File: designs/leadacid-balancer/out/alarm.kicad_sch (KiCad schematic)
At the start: 1 part, among them J2 1757242

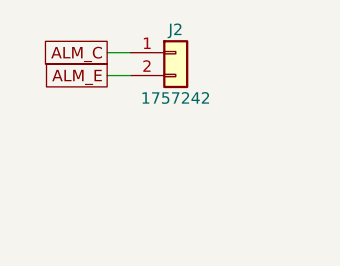
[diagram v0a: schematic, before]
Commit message: designs: work-in-progress (review fixes under way)
Co-Authored-By: Claude Opus 5.5 <noreply@anthropic.com>
Claude-Session: https://claude.ai/code/session_01VFJn9VbX8h27kf4LpLwEtn
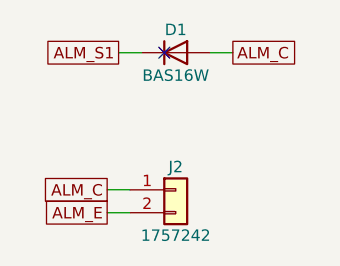
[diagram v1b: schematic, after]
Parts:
- added D1: BAS16W, Package_TO_SOT_SMD:SOT-323_SC-70, symbol Diode:BAS16W
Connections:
- net ALM_C: now also D1.1 (A)
- new net ALM_S1: D1.3 (K)
- no-connect marks 0 -> 1
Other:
- moved on the sheet: J2
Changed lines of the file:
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@@
 		(rev "A")
 		(company "kaesynth")
-		(comment 1 "J2 = MSTBA 2-pos: 1 ALM_C, 2 ALM_E; U110/U210/U310 collectors in parallel")
+		(comment 1 "J2 = MSTBA 2-pos: 1 ALM_C, 2 ALM_E; D1 blocks a reversed loop (review MINOR-9); U110, U210, U310 outputs in series: closed = healthy (fail-safe)")
 		(comment 2 "Lead-acid string balancer, 2:1 switched capacitor, 2-4 x 12 V — generated by kaesynth from design.py; do not edit by hand")
 	)
 	(symbol
 		(lib_id "Connector_Generic:Conn_01x02")
+		(at 43.18 45.72 0)
+		(unit 1)
+		(exclude_from_sim no)
+		(in_bom yes)
+		(on_board yes)
+		(dnp no)
+		(property "Reference" "J2"
+			(at 43.18 43.18 0)
+			(effects
+				(font (size 1.27 1.27))
+			)
+		)
+		(property "Value" "1757242"
+			(at 43.18 50.8 0)
+			(effects
+				(font (size 1.27 1.27))
+			)
+		)
+		(property "Footprint" "Connector_Phoenix_MSTB:PhoenixContact_MSTBA_2,5_2-G-5,08_1x02_P5.08mm_Horizontal"
+			(at 43.18 45.72 0)
+			(hide yes)
+			(effects
+				(font (size 1.27 1.27))
+			)
+		)
+		(property "Datasheet" "https://www.phoenixcontact.com/en-us/products/pcb-header-mstba-25-2-g-508-1757242"
+			(at 43.18 45.72 0)
+			(hide yes)
+			(effects
+				(font (size 1.27 1.27))
+			)
+		)
+		(property "Description" "PCB header MSTBA 2,5/2-G-5,08, 2 pos (isolated alarm contact)"
+			(at 43.18 45.72 0)
+			(hide yes)
+			(effects
+				(font (size 1.27 1.27))
+			)
+		)
+		(property "MPN" "1757242"
+			(at 43.18 45.72 0)
+			(hide yes)
+			(effects
+				(font (size 1.27 1.27))
+			)
+		)
+		(property "Manufacturer" "Phoenix Contact"
+			(at 43.18 45.72 0)
+			(hide yes)
+			(effects
+				(font (size 1.27 1.27))
+			)
+		)
+		(property "Block" "alarm"
+			(at 43.18 45.72 0)
+			(hide yes)
+			(effects
+				(font (size 1.27 1.27))
+			)
+		)
+		(property "Component Class" "alarm"
+			(at 43.18 45.72 0)
+			(hide yes)
+			(effects
+				(font (size 1.27 1.27))
+			)
+		)
+		(pin "1"
+		)
+		(pin "2"
+		)
+		(instances
+			(project "leadacid-balancer"
+				(path "/19cb7a1a-0065-5673-9954-2860fa0f563d/cf1d326d-1904-5168-b9da-d8ce55ede38b"
+					(reference "J2")
+					(unit 1)
+				)
+			)
+		)
+	)
+	(wire
+		(pts (xy 38.1 45.72) (xy 35.56 45.72))
+		(stroke
+			(width 0)
+			(type default)
+		)
+	)
+	(global_label "ALM_C"
+		(shape passive)
+		(at 35.56 45.72 180)
+		(fields_autoplaced yes)
+		(effects
+			(font (size 1.27 1.27))
+			(justify right)
+		)
+		(property "Intersheetrefs" "${INTERSHEET_REFS}"
+			(at 35.56 45.72 0)
+			(hide yes)
+			(effects
+				(font (size 1.27 1.27))
+			)
+		)
+	)
+	(wire
+		(pts (xy 38.1 48.26) (xy 35.56 48.26))
+		(stroke
+			(width 0)
+			(type default)
+		)
+	)
+	(global_label "ALM_E"
+		(shape passive)
+		(at 35.56 48.26 180)
+		(fields_autoplaced yes)
+		(effects
+			(font (size 1.27 1.27))
+			(justify right)
+		)
+		(property "Intersheetrefs" "${INTERSHEET_REFS}"
+			(at 35.56 48.26 0)
+			(hide yes)
+			(effects
+				(font (size 1.27 1.27))
+			)
+		)
+	)
+	(symbol
+		(lib_id "Diode:BAS16W")
 		(at 43.18 30.48 0)
 		(unit 1)
@@
 		(on_board yes)
 		(dnp no)
-		(property "Reference" "J2"
+		(property "Reference" "D1"
 			(at 43.18 27.94 0)
 			(effects
@@
 			)
 		)
-		(property "Value" "1757242"
-			(at 43.18 35.56 0)
-			(effects
-				(font (size 1.27 1.27))
-			)
-		)
-		(property "Footprint" "Connector_Phoenix_MSTB:PhoenixContact_MSTBA_2,5_2-G-5,08_1x02_P5.08mm_Horizontal"
-			(at 43.18 30.48 0)
-			(hide yes)
-			(effects
-				(font (size 1.27 1.27))
-			)
-		)
-		(property "Datasheet" "https://www.phoenixcontact.com/en-us/products/pcb-header-mstba-25-2-g-508-1757242"
-			(at 43.18 30.48 0)
-			(hide yes)
-			(effects
-				(font (size 1.27 1.27))
-			)
-		)
-		(property "Description" "PCB header MSTBA 2,5/2-G-5,08, 2 pos (isolated alarm contact)"
-			(at 43.18 30.48 0)
-			(hide yes)
-			(effects
-				(font (size 1.27 1.27))
-			)
-		)
-		(property "MPN" "1757242"
-			(at 43.18 30.48 0)
-			(hide yes)
-			(effects
-				(font (size 1.27 1.27))
-			)
-		)
-		(property "Manufacturer" "Phoenix Contact"
+		(property "Value" "BAS16W"
+			(at 43.18 33.02 0)
+			(effects
+				(font (size 1.27 1.27))
+			)
+		)
+		(property "Footprint" "Package_TO_SOT_SMD:SOT-323_SC-70"
+			(at 43.18 30.48 0)
+			(hide yes)
+			(effects
+				(font (size 1.27 1.27))
+			)
+		)
+		(property "Datasheet" "https://www.diodes.com/assets/Datasheets/ds30117.pdf"
+			(at 43.18 30.48 0)
+			(hide yes)
+			(effects
+				(font (size 1.27 1.27))
+			)
+		)
+		(property "Description" "Switching diode 75 V 150 mA SOT-323 (bootstrap)"
+			(at 43.18 30.48 0)
+			(hide yes)
+			(effects
+				(font (size 1.27 1.27))
+			)
+		)
+		(property "MPN" "BAS16W-7-F"
+			(at 43.18 30.48 0)
+			(hide yes)
+			(effects
+				(font (size 1.27 1.27))
+			)
+		)
+		(property "Manufacturer" "Diodes Incorporated"
 			(at 43.18 30.48 0)
 			(hide yes)
@@
 		)
 		(pin "2"
+		)
+		(pin "3"
 		)
 		(instances
 			(project "leadacid-balancer"
 				(path "/19cb7a1a-0065-5673-9954-2860fa0f563d/cf1d326d-1904-5168-b9da-d8ce55ede38b"
-					(reference "J2")
+					(reference "D1")
 					(unit 1)
 				)
@@
 	)
 	(wire
-		(pts (xy 38.1 30.48) (xy 35.56 30.48))
+		(pts (xy 46.99 30.48) (xy 49.53 30.48))
 		(stroke
 			(width 0)
@@
 	(global_label "ALM_C"
 		(shape passive)
-		(at 35.56 30.48 180)
+		(at 49.53 30.48 0)
+		(fields_autoplaced yes)
+		(effects
+			(font (size 1.27 1.27))
+			(justify left)
+		)
+		(property "Intersheetrefs" "${INTERSHEET_REFS}"
+			(at 49.53 30.48 0)
+			(hide yes)
+			(effects
+				(font (size 1.27 1.27))
+			)
+		)
+	)
+	(no_connect
+		(at 41.91 30.48)
+	)
+	(wire
+		(pts (xy 39.37 30.48) (xy 36.83 30.48))
+		(stroke
+			(width 0)
+			(type default)
+		)
+	)
+	(global_label "ALM_S1"
+		(shape passive)
+		(at 36.83 30.48 180)
 		(fields_autoplaced yes)
 		(effects
@@
 		)
 		(property "Intersheetrefs" "${INTERSHEET_REFS}"
-			(at 35.56 30.48 0)
-			(hide yes)
-			(effects
-				(font (size 1.27 1.27))
-			)
-		)
-	)
-	(wire
-		(pts (xy 38.1 33.02) (xy 35.56 33.02))
-		(stroke
-			(width 0)
-			(type default)
-		)
-	)
-	(global_label "ALM_E"
-		(shape passive)
-		(at 35.56 33.02 180)
-		(fields_autoplaced yes)
-		(effects
-			(font (size 1.27 1.27))
-			(justify right)
-		)
-		(property "Intersheetrefs" "${INTERSHEET_REFS}"
-			(at 35.56 33.02 0)
-			(hide yes)
-			(effects
+			(at 36.83 30.48 0)
+			(hide yes)
+			(effects
